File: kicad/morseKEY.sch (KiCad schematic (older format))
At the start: 14 parts, among them P1 USB_A, P2 KEY, P3 ISP, U1 ATTINY85-P

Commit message: 3D render
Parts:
- R4: footprint morseKEY:Pin_Header_Straight_1x03 -> morseKEY:res_vert
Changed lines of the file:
@@
 F 0 "R4" H 3200 2875 50  0000 C CNB
 F 1 "2k5" V 3300 2875 50  0000 C CNN
-F 2 "morseKEY:Pin_Header_Straight_1x03" V 3230 2875 50  0001 C CNN
+F 2 "morseKEY:res_vert" V 3230 2875 50  0001 C CNN
 F 3 "" H 3300 2875 50  0000 C CNN
 F 4 "mfr_pn" H 3300 2875 60  0001 C CNN "manf#"

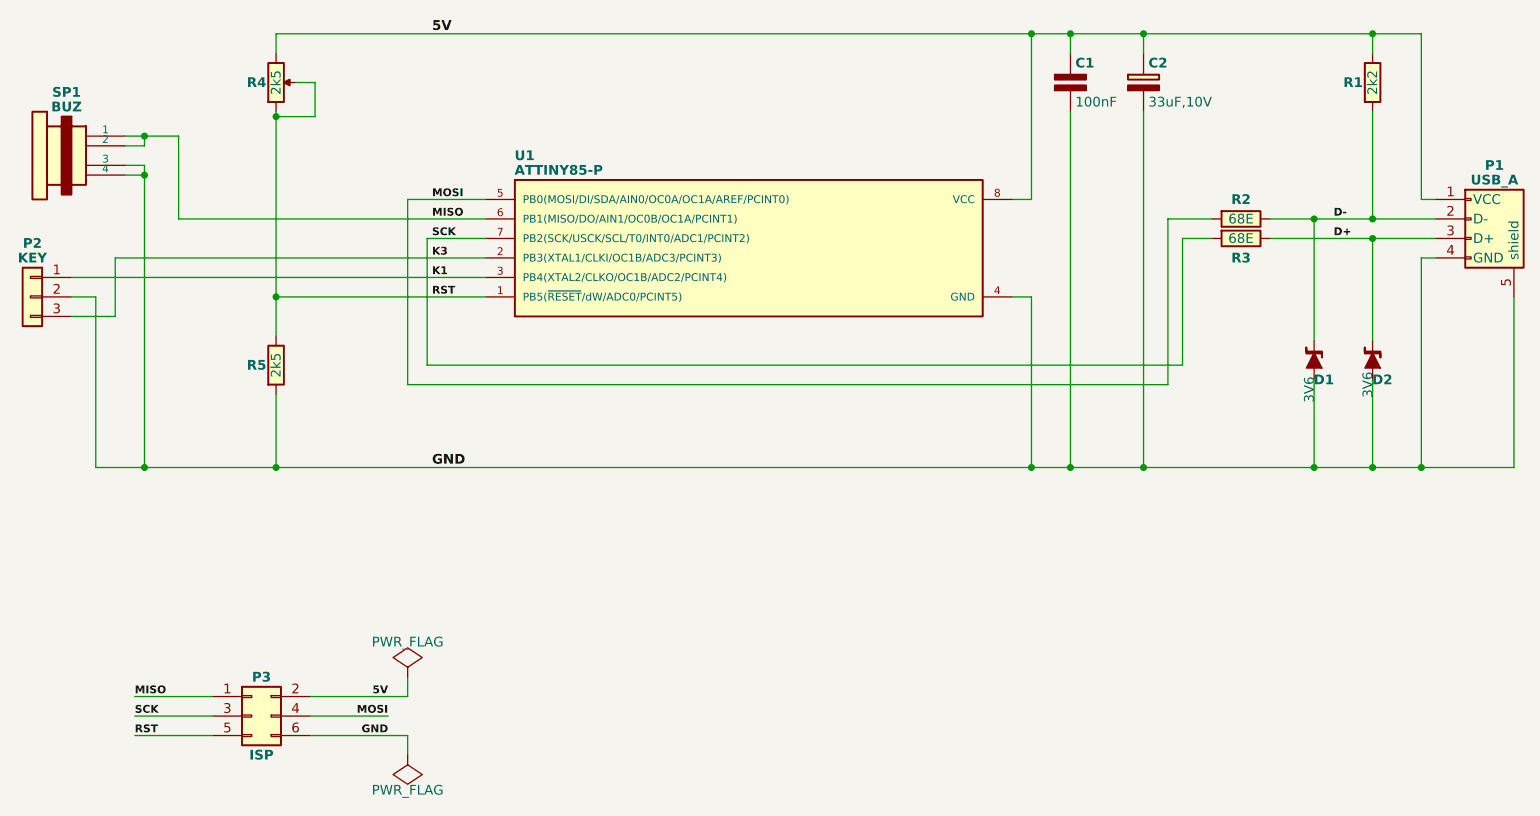
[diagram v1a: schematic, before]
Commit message: board layout
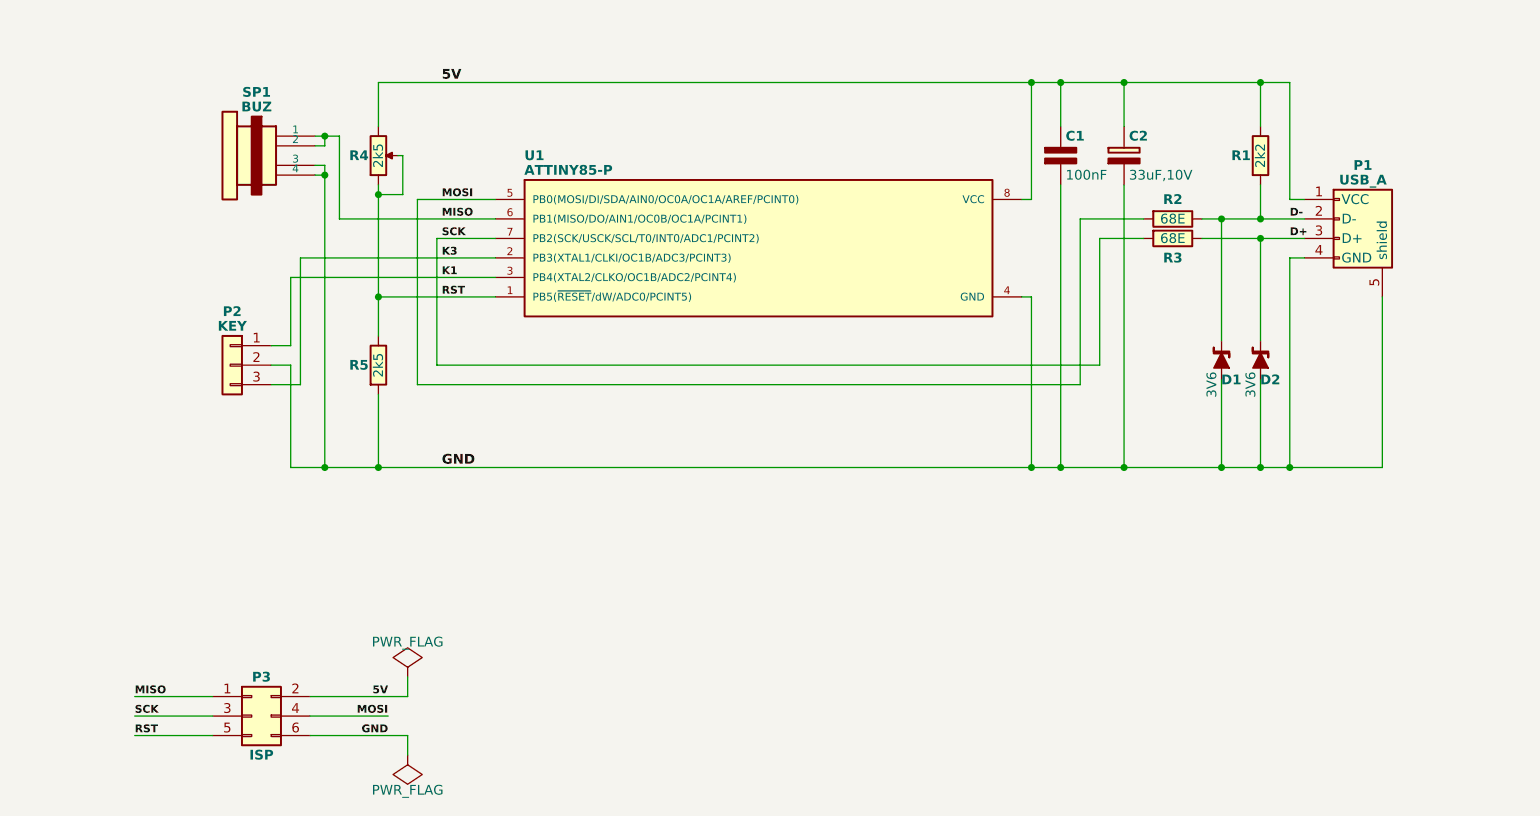
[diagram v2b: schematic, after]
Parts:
- P1: footprint morseKEY:USB_A -> morseKEY:USB_A_up2-ah-th
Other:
- moved on the sheet: C1, C2, D1, D2, P1, P2, R1, R2, R3, R4, R5, SP1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
